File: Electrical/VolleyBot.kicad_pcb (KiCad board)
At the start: 2 copper layers, 95.2 x 57.5 mm, 66 parts, among them J1 Conn_01x04_Pin, J2 Conn_01x04_Pin, J3 Conn_01x02_Pin, J4 Conn_01x04_Socket, J5 Conn_01x02_Socket, J6 Conn_01x02_Socket, J7 Conn_01x02_Socket, SW1 SW_SPDT, U1 STM32F411CEU6, U2 DRV8833PWP, U3 DRV8833PWP, U4 AP62300TWU, U5 AP62300TWU, Y1 16MHz

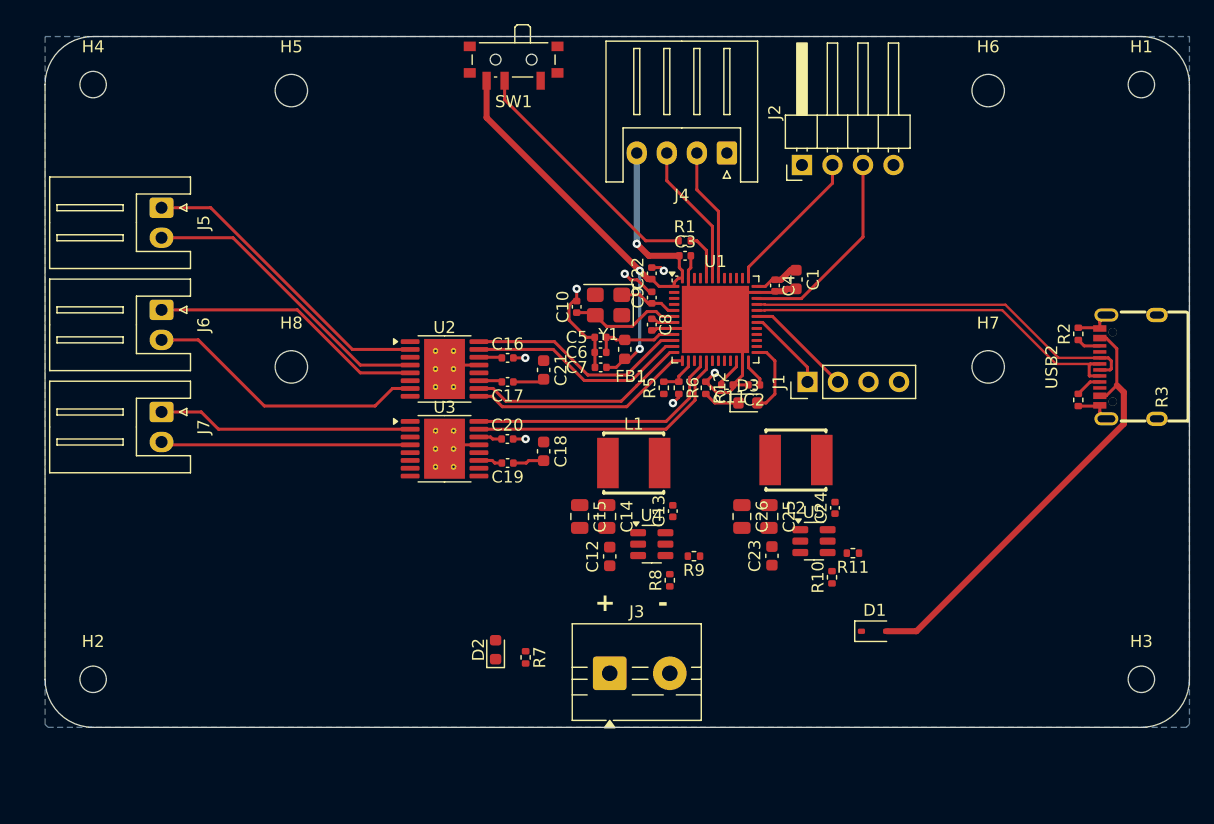
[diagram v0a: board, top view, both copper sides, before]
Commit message: routed pcb
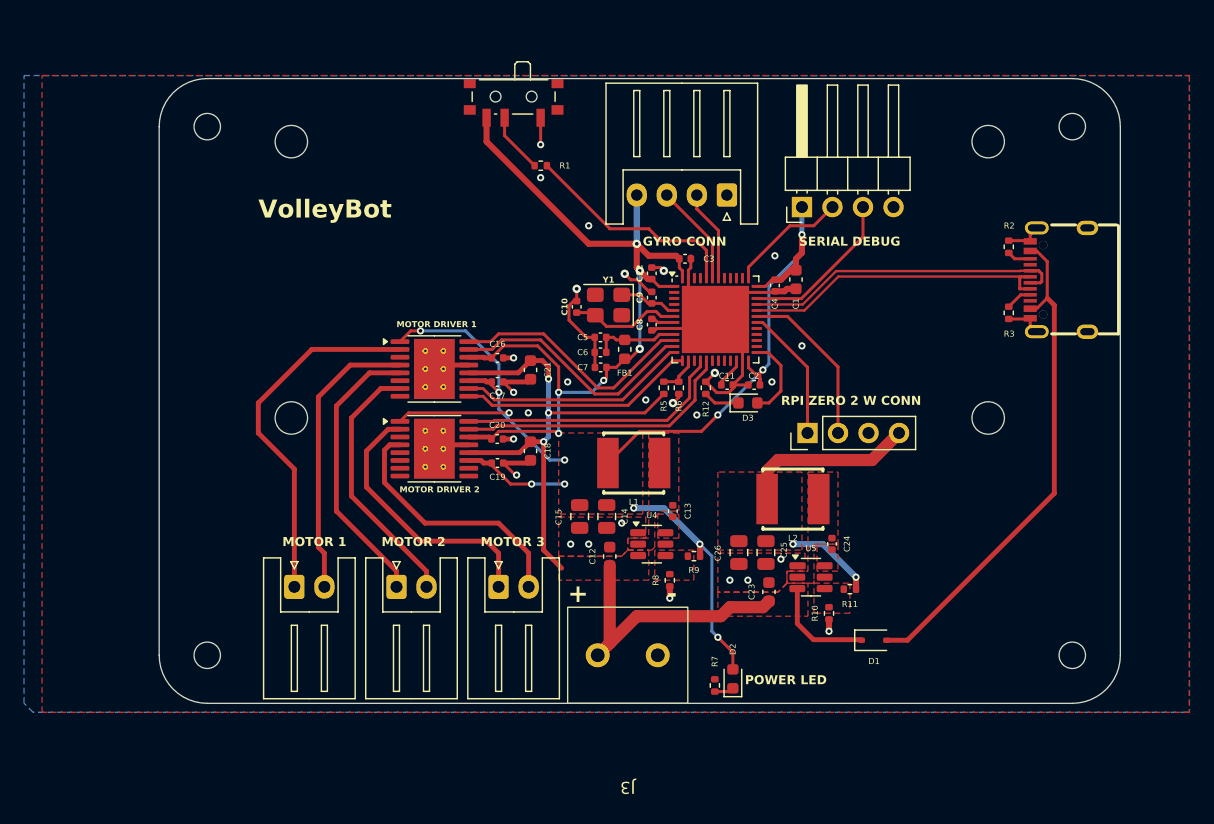
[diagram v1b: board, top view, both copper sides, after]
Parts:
- J3: footprint TerminalBlock:TerminalBlock_MaiXu_MX126-5.0-02P_1x02_P5.00mm -> Rocketry_Manual:Screw_Terminal_2_Pins
- moved J5 33.4 mm to (84.8, 106.6), turned to 0 degrees
- moved J7 31.6 mm to (101.8, 106.6), turned to 0 degrees
- moved J6 30.2 mm to (93.2, 106.6), turned to 0 degrees
- moved D2 19.9 mm to (121.2, 114.2)
- moved R7 15.9 mm to (119.8, 114.8)
- moved R1 13.5 mm to (105.3, 71.5)
- moved H4 10.1 mm to (77.5, 68.2)
- moved H2 9.71 mm to (77.5, 112.2)
- moved R2 9.28 mm to (144.2, 78.2)
- moved R3 9.28 mm to (144.2, 83.8)
- moved USB2 9.28 mm to (148.4, 81.0)
- moved H1 6.73 mm to (149.5, 68.2)
- moved H3 6.09 mm to (149.5, 112.2)
- moved H5 4.25 mm to (84.5, 69.5)
- moved H6 4.25 mm to (142.5, 69.5)
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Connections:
- C18 pad 1: /VBATT -> +BATT
- C21 pad 1: /VBATT -> +BATT
- U2 pad 12: /VBATT -> +BATT
- U3 pad 12: /VBATT -> +BATT
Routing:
- net +3.3V: track 63.1 -> 174.1 mm, vias 3 -> 18
- net +BATT: track 0.00 -> 73.0 mm, vias 0 -> 3
- net +5V: track 0.00 -> 21.8 mm, vias 0 -> 2
- net Net-(SW1-B): track 20.9 -> 5.65 mm
- net /BOOT0: track 3.94 -> 18.5 mm
- net -BATT: track 64.7 -> 71.2 mm, vias 7 -> 27
- net /USB_D-: track 33.1 -> 26.6 mm
- net /USB_D+: track 33.1 -> 26.6 mm
- net VBUS: track 37.0 -> 42.1 mm
- net /USART1_RX: track 9.02 -> 14.0 mm
- net Net-(J5-Pin_1): track 25.6 -> 29.9 mm
- net /USART1_TX: track 6.99 -> 11.2 mm
- net Net-(J4-Pin_2): track 11.2 -> 7.66 mm
- net Net-(J4-Pin_3): track 12.0 -> 8.49 mm
- net /SWDIO: track 17.0 -> 13.5 mm
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- added copper zone on F.Cu, net +3.3V
- added copper zone on F.Cu, net +5V
- added copper zone on F.Cu, net +BATT
- added copper zone on F.Cu, net -BATT
- added copper zone on F.Cu, net /BST1
- added copper zone on F.Cu, net /BST2
- added copper zone on F.Cu, net /FB1
- added copper zone on F.Cu, net /FB2
- added copper zone on F.Cu, net /SW1
- added copper zone on F.Cu, net /SW2
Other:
- board size 95.2 x 57.5 mm -> 80 x 52 mm
- board text added: "GYRO CONN"
- board text added: "MOTOR 1"
- board text added: "MOTOR 2"
- board text added: "MOTOR 3"
- board text added: "MOTOR DRIVER 1"
- board text added: "MOTOR DRIVER 2"
- board text added: "POWER LED"
- board text added: "RPI ZERO 2 W CONN"
- board text added: "SERIAL DEBUG"
- board text added: "VolleyBot"
